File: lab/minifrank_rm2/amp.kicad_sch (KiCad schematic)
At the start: 20 parts, among them U2 LM358

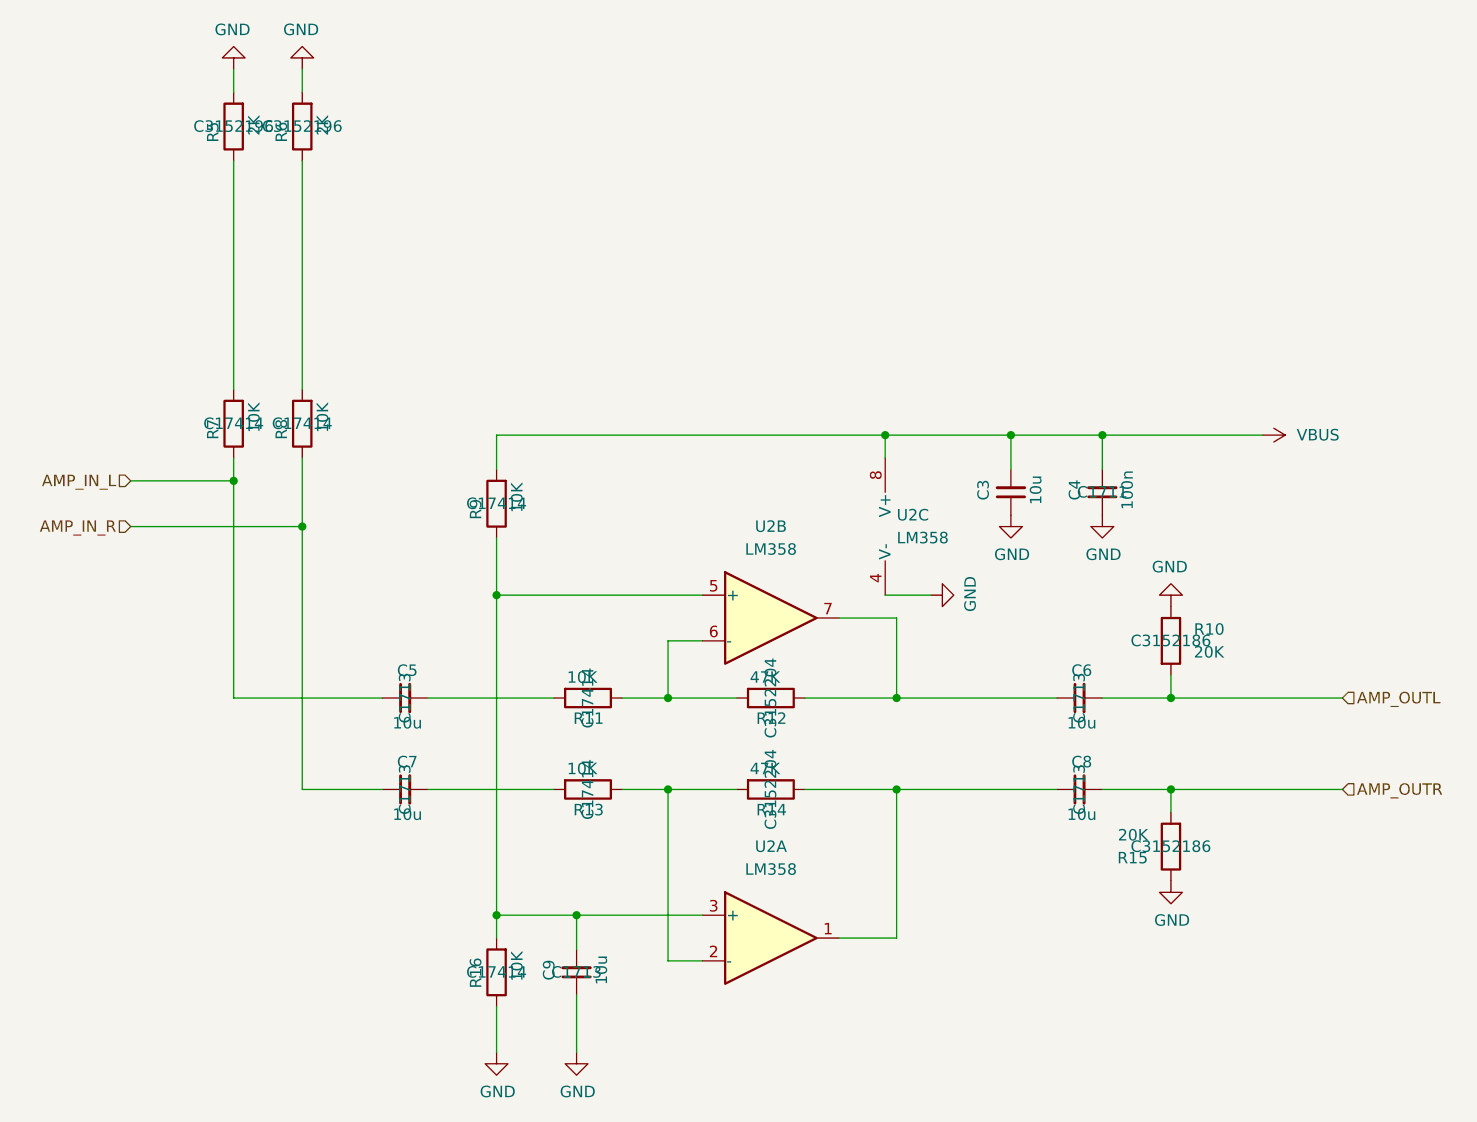
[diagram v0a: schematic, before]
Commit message: MiniFRANK RM2 1.02
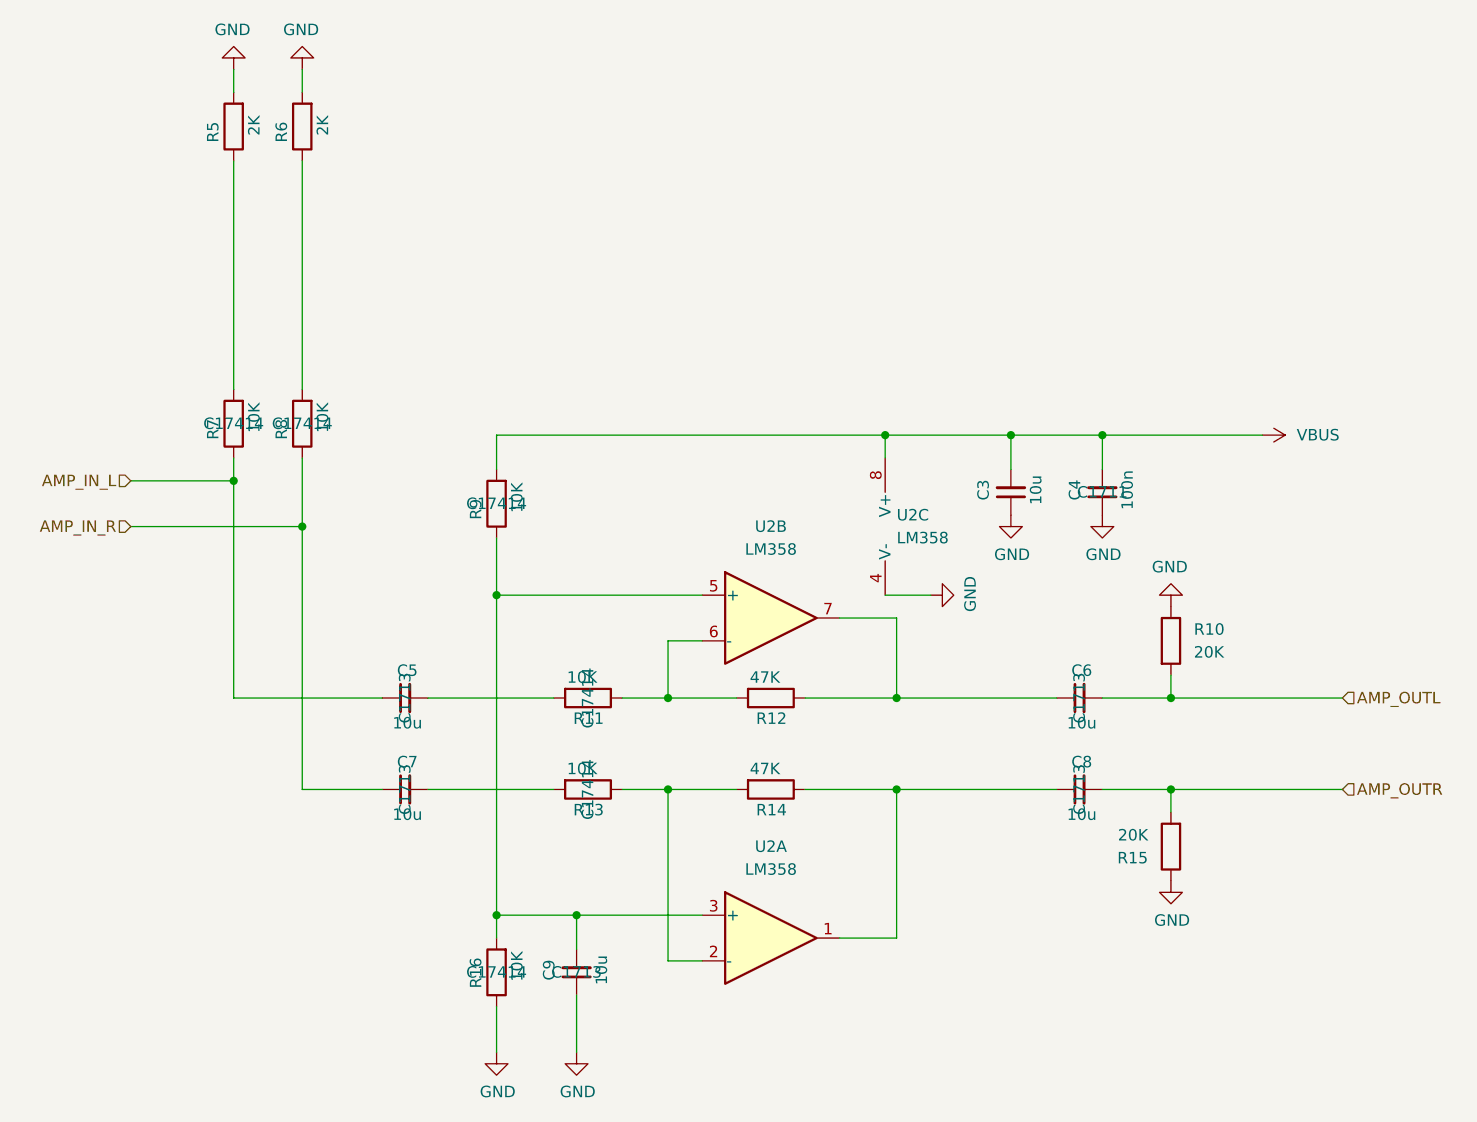
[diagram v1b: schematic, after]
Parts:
- R10, R15: LCSC C3152186 -> (none)
- R12, R14: LCSC C3152204 -> (none)
- R5, R6: LCSC C3152196 -> (none)
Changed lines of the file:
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@@
 			)
 		)
-		(property "LCSC" "C3152186"
+		(property "LCSC" ""
 			(at 199.39 129.54 0)
 			(effects
@@
 			)
 		)
-		(property "LCSC" "C3152196"
+		(property "LCSC" ""
 			(at 95.25 49.53 0)
 			(effects
@@
 			)
 		)
-		(property "LCSC" "C3152204"
+		(property "LCSC" ""
 			(at 154.94 113.03 0)
 			(effects
@@
 			)
 		)
-		(property "LCSC" "C3152204"
+		(property "LCSC" ""
 			(at 154.94 123.19 0)
 			(effects
@@
 			)
 		)
-		(property "LCSC" "C3152186"
+		(property "LCSC" ""
 			(at 199.39 106.68 0)
 			(effects
@@
 			)
 		)
-		(property "LCSC" "C3152196"
+		(property "LCSC" ""
 			(at 102.87 49.53 0)
 			(effects
